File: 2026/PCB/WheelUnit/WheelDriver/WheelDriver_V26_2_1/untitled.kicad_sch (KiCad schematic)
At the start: 68 parts, among them J1 Conn_01x07_Pin, J4 Conn_01x03_Socket, J5 Conn_01x02_Socket, SW1 SW_MEC_5E, SW2 SW_MEC_5E, U1 MAX3051

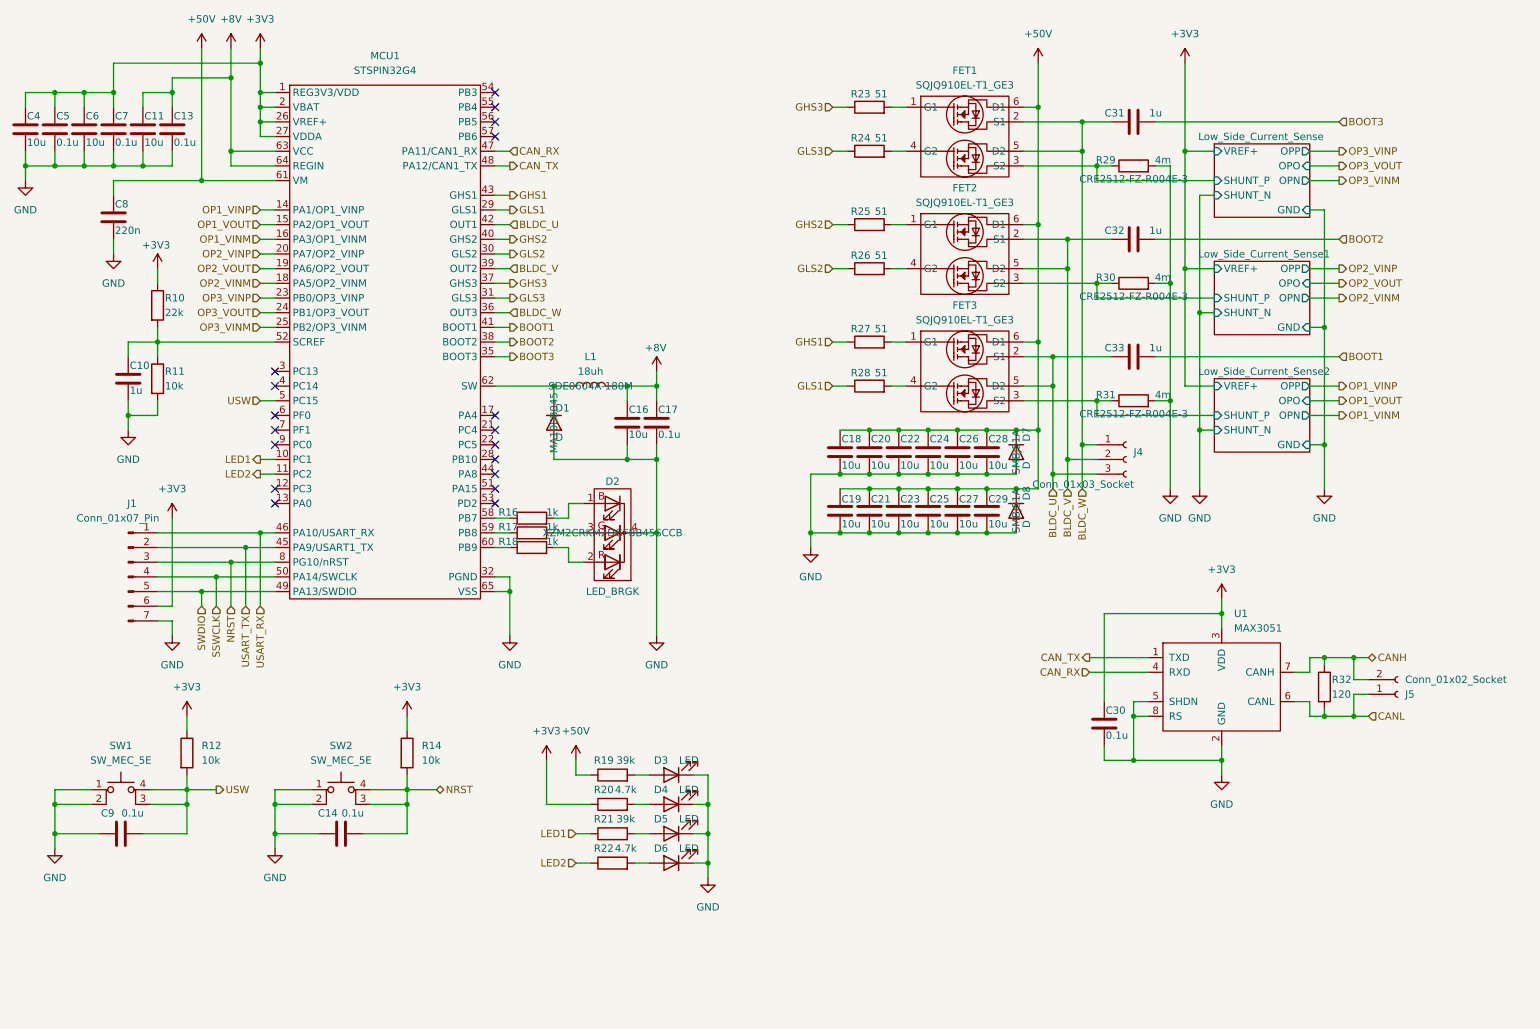
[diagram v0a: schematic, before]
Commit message: 回路図4ch化
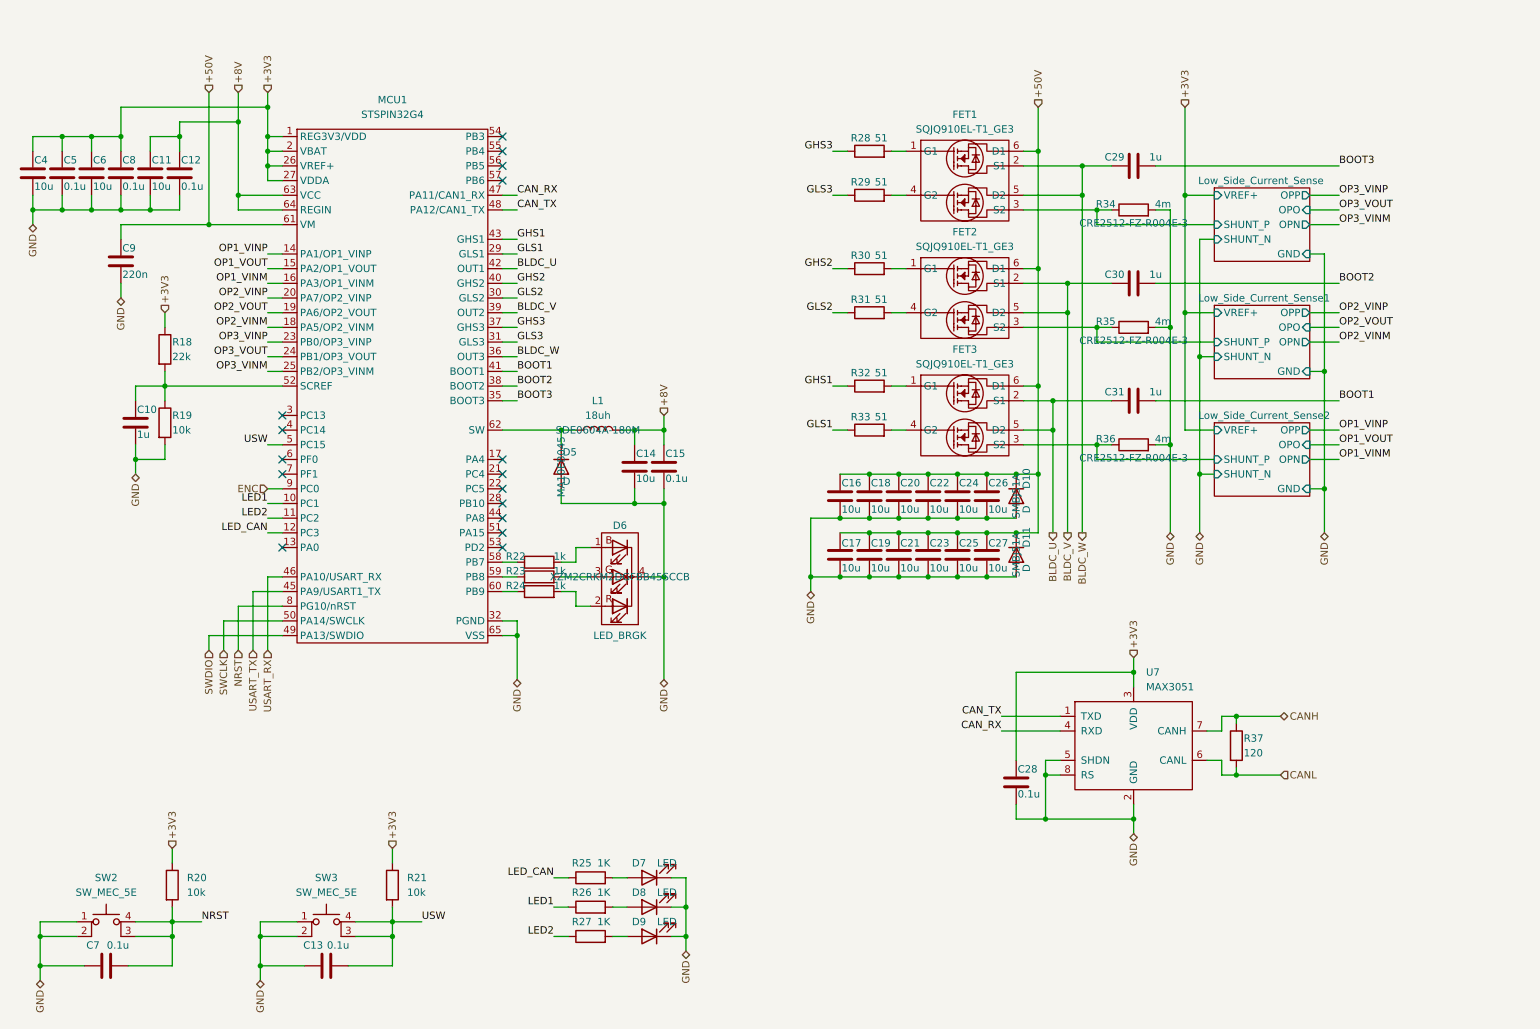
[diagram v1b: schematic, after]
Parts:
- removed D3: LED, BLDCUint_LIB_FTP:LED_1608_user_dif, symbol Device:LED
- removed FET1, FET2, FET3: SQJQ910EL-T1_GE3, BLDCUint_LIB_FTP:SQJQ910EL-T1_GE3, symbol BLDCUnit_LIB_SYM:SQJQ910EL-T1_GE3
- removed J1: Conn_01x07_Pin, Connector_JST:JST_PH_S7B-PH-K_1x07_P2.00mm_Horizontal, symbol Connector:Conn_01x07_Pin
- removed J4: Conn_01x03_Socket, Connector_Molex:Molex_SPOX_5268-03A_1x03_P2.50mm_Horizontal, symbol Connector:Conn_01x03_Socket
- removed J5: Conn_01x02_Socket, Connector_JST:JST_PH_S2B-PH-K_1x02_P2.00mm_Horizontal, symbol Connector:Conn_01x02_Socket
- removed R19: 39k, Resistor_SMD:R_0402_1005Metric_Pad0.72x0.64mm_HandSolder, symbol Device:R
- added FET1, FET2, FET3: SQJQ910EL-T1_GE3, symbol WheelUnit_LIB_SYM:SQJQ910EL-T1_GE3
- R25: renamed from R20; value 4.7k -> 1K
- R26: renamed from R21; value 39k -> 1K
- R27: renamed from R22; value 4.7k -> 1K
- renumbered C13 to C12, C14 to C13, C16 to C14, C17 to C15, C18 to C16, C19 to C17, C20 to C18, C21 to C19, C22 to C20, C23 to C21, C24 to C22, C25 to C23, C26 to C24, C27 to C25, C28 to C26, C29 to C27, C30 to C28, C31 to C29, C32 to C30, C33 to C31, C9 to C7, C7 to C8, C8 to C9, D7 to D10, D8 to D11, D1 to D5, D2 to D6, D4 to D7, D5 to D8, D6 to D9, R10 to R18, R11 to R19, R12 to R20, R14 to R21, R16 to R22, R17 to R23, R18 to R24, R23 to R28, R24 to R29, R25 to R30, R26 to R31, R27 to R32, R28 to R33, R29 to R34, R30 to R35, R31 to R36, R32 to R37, SW1 to SW2, SW2 to SW3, U1 to U7
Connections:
- net +3V3: no longer R25.1
- net +50V: now also FET1.6 (D1), FET2.6 (D1), FET3.6 (D1)
- net BLDC_U: now also FET3.2 (S1), FET3.5 (D2)
- net BLDC_V: now also FET2.2 (S1), FET2.5 (D2)
- net BLDC_W: now also FET1.2 (S1), FET1.5 (D2)
- net Low_Side_Current_Sense/SHUNT_P: now also FET1.3 (S2)
- net Low_Side_Current_Sense1/SHUNT_P: now also FET2.3 (S2)
- net Low_Side_Current_Sense2/SHUNT_P: now also FET3.3 (S2)
- net NRST: now also C7.1, R20.2, SW2.3 (K), SW2.4 (A); no longer C13.1, R21.2, SW3.3 (K), SW3.4 (A)
- net USW: now also C13.1, R21.2, SW3.3 (K), SW3.4 (A); no longer C7.1, R20.2, SW2.3 (K), SW2.4 (A)
- net at R31.2: now also FET2.4 (G2)
- net at R32.2: now also FET3.1 (G1)
- net at R33.2: now also FET3.4 (G2)
- net at R28.2: now also FET1.1 (G1)
- net at R29.2: now also FET1.4 (G2)
- net at R30.2: now also FET2.1 (G1)
- net LED_CAN: now reaches MCU1.12 (PC3)
- net LED_CAN: now also R25.1
- net ENC: now reaches MCU1.9 (PC0)
- net SSWCLK renamed SWCLK
- no-connect marks 18 -> 16
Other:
- moved on the sheet: C10, C11, C12, C13, C14, C15, C16, C17, C18, C19, C20, C21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
